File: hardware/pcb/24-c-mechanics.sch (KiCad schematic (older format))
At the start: 22 parts, among them U301 VID28-05, U302 VID66-08, U303 AH3572, U304 AH3572

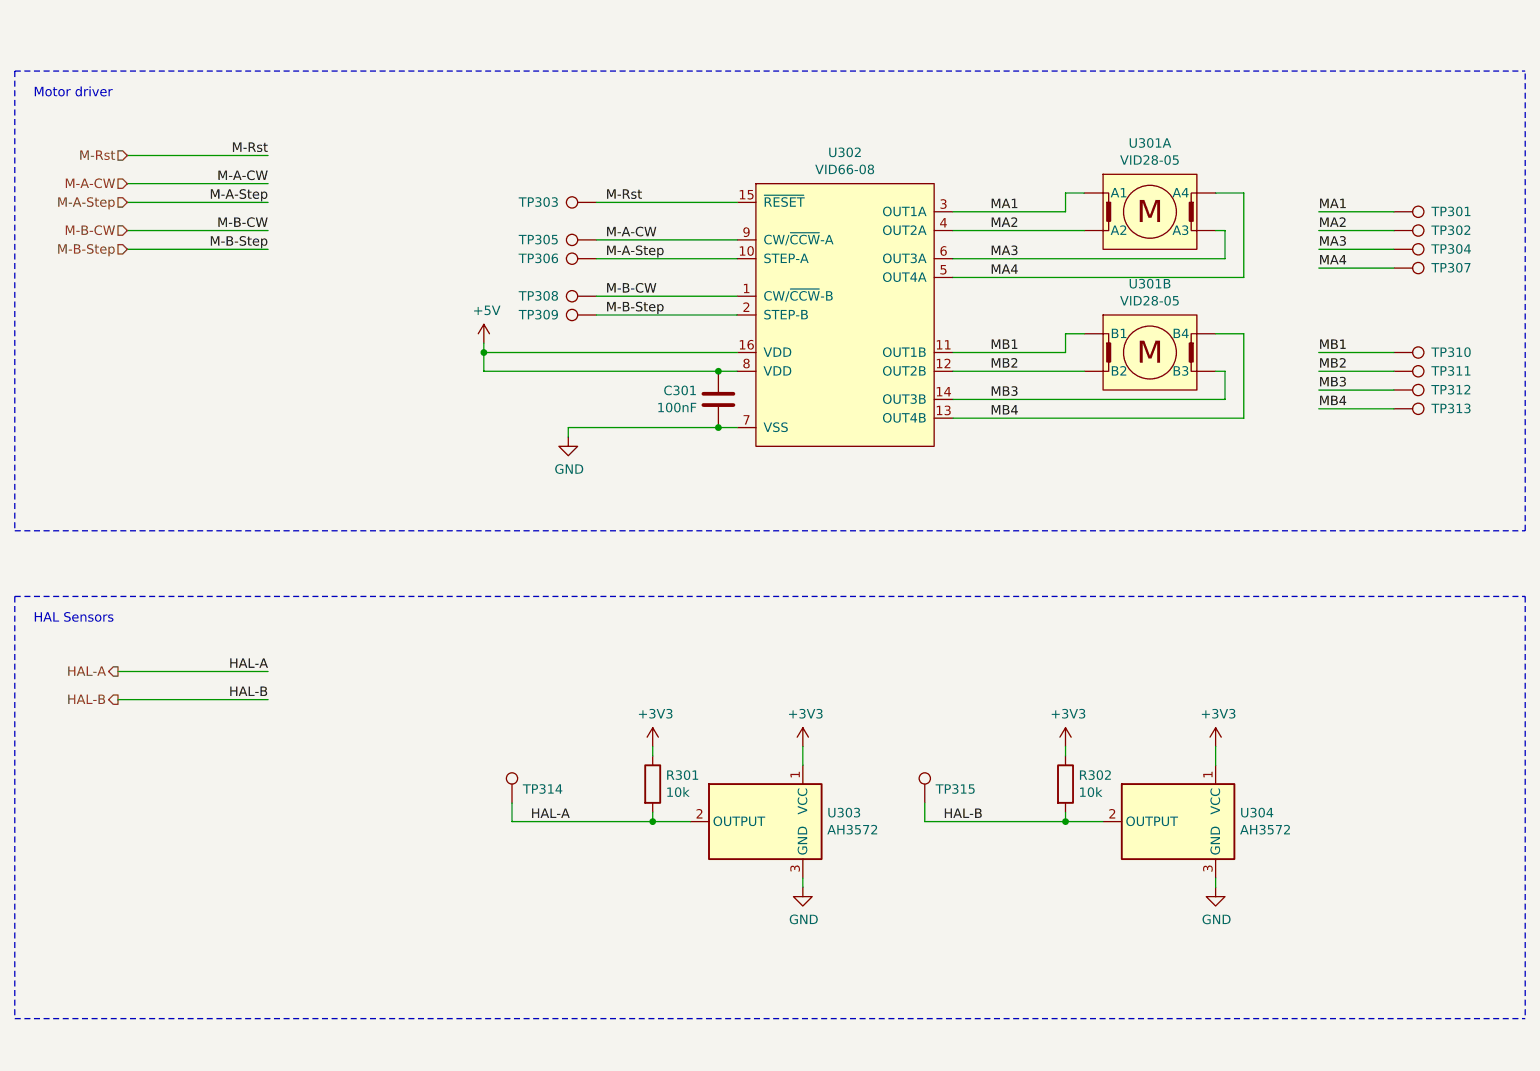
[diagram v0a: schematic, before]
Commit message: Finished PCB (#3)
* Created PCB outline and first placement

* Changed connectors

* Minor

* Included all 3D files

* Mixed changes

* Changed supply to 7V

* Archived PCB project

* Update 24-clocks-rescue.lib

* First placement

* Routed supplies

* Update 24-clocks.kicad_pcb

* Added routing

* Routed more nets

* Finished routing

* Archived project

* Replace hash and date

* minor

* Update pcb.yml

* Update pcb.yml

* Update pcb.yml

* Update pcb.yml

* Auto update commit date and hash

* Update output

* changed outputs

* Added layer to output

* Update hash and date also in sch

* Added caps to hall sensors

* Cleanup files
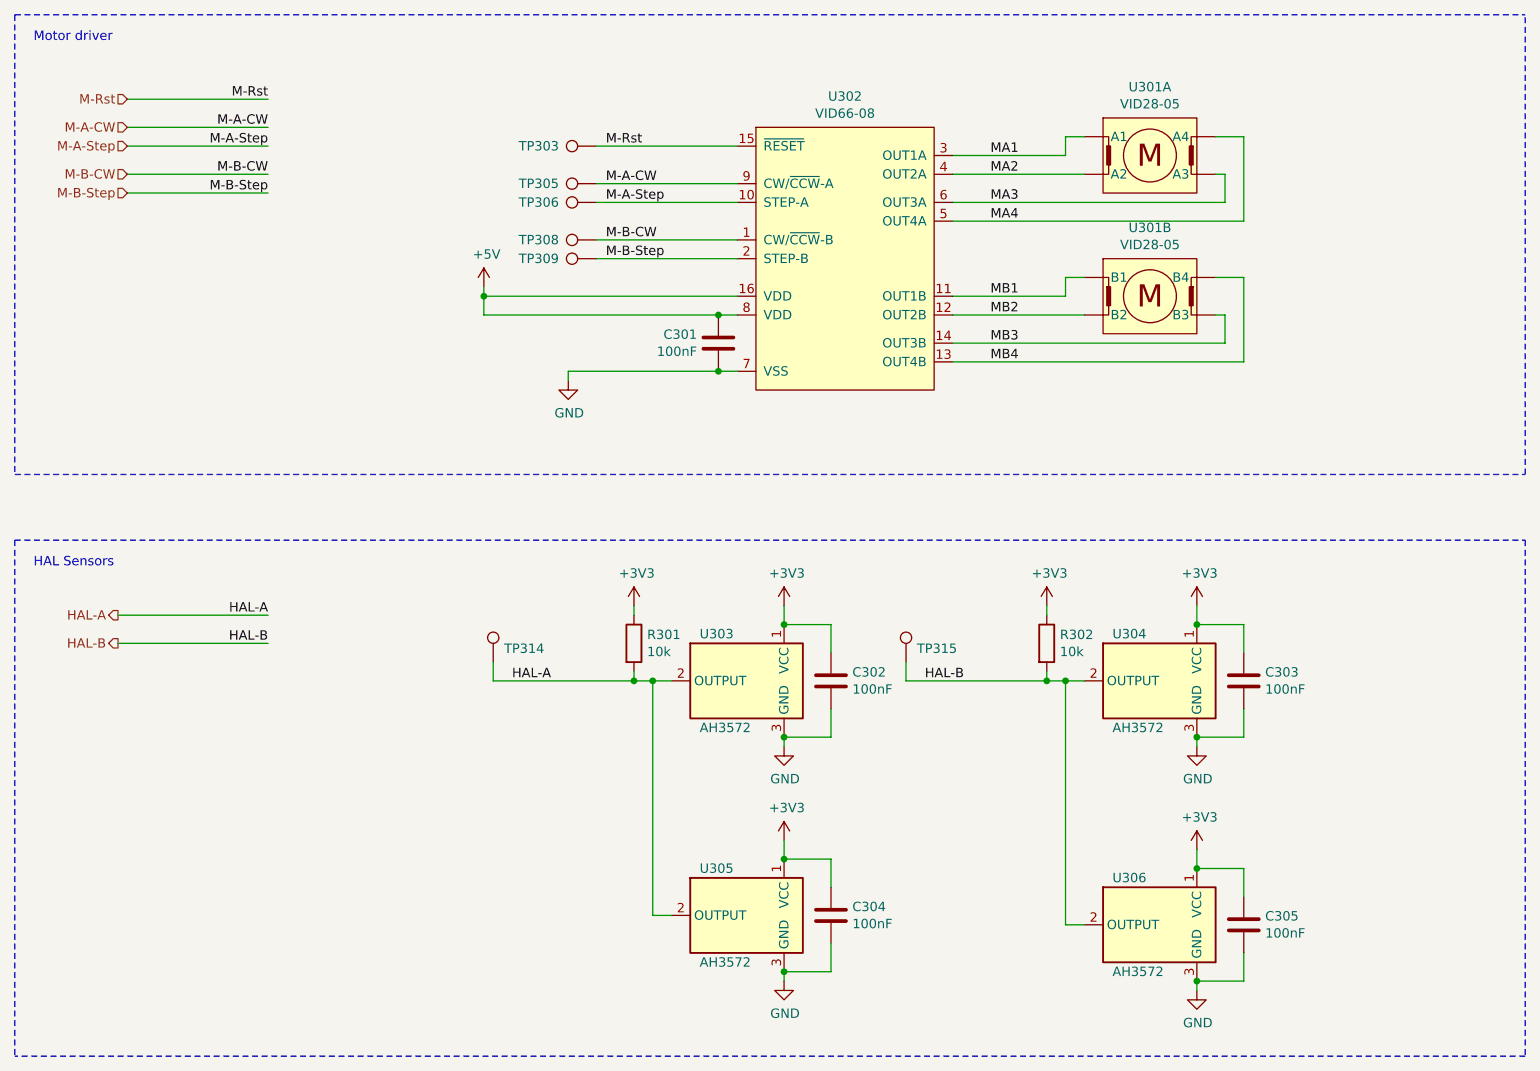
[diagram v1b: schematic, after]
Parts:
- removed TP301: MA1, TestPoint:TestPoint_Pad_D2.0mm, symbol Connector:TestPoint
- removed TP302: MA2, TestPoint:TestPoint_Pad_D2.0mm, symbol Connector:TestPoint
- removed TP304: MA3, TestPoint:TestPoint_Pad_D2.0mm, symbol Connector:TestPoint
- removed TP307: MA4, TestPoint:TestPoint_Pad_D2.0mm, symbol Connector:TestPoint
- removed TP310: MB1, TestPoint:TestPoint_Pad_D2.0mm, symbol Connector:TestPoint
- removed TP311: MB2, TestPoint:TestPoint_Pad_D2.0mm, symbol Connector:TestPoint
- removed TP312: MB3, TestPoint:TestPoint_Pad_D2.0mm, symbol Connector:TestPoint
- removed TP313: MB4, TestPoint:TestPoint_Pad_D2.0mm, symbol Connector:TestPoint
- added C302, C303, C304, C305: 100nF, Capacitor_SMD:C_0603_1608Metric, symbol Device:C
- added U305, U306: AH3572, Package_TO_SOT_SMD:TSOT-23, symbol Sensor_Magnetic:SM351LT
- U301: footprint mvl-footprints:vid_28_05 -> mvl-footprints:BK30D-R5
- U303, U304: footprint Package_TO_SOT_SMD:SOT-23 -> mvl-footprints:SOT-23-UD; Config -MASTER -> -MASTER,-SLAVE
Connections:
- net +3V3: now also C302.2, C303.2, C304.2, C305.2, U305.1 (VCC), U306.1 (VCC)
- net GND: now also C302.1, C303.1, C304.1, C305.1, U305.3 (GND), U306.3 (GND)
- net HAL-A: now also U305.2 (OUTPUT)
- net HAL-B: now also U306.2 (OUTPUT)
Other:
- moved on the sheet: C301, R301, R302, TP303, TP305, TP306, TP308, TP309, TP314, TP315, U301A, U301B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
